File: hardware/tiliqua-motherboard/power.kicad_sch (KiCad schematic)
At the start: 23 parts, among them J6 CONN 2x5 P=2.54mm, U5 AP63200WU

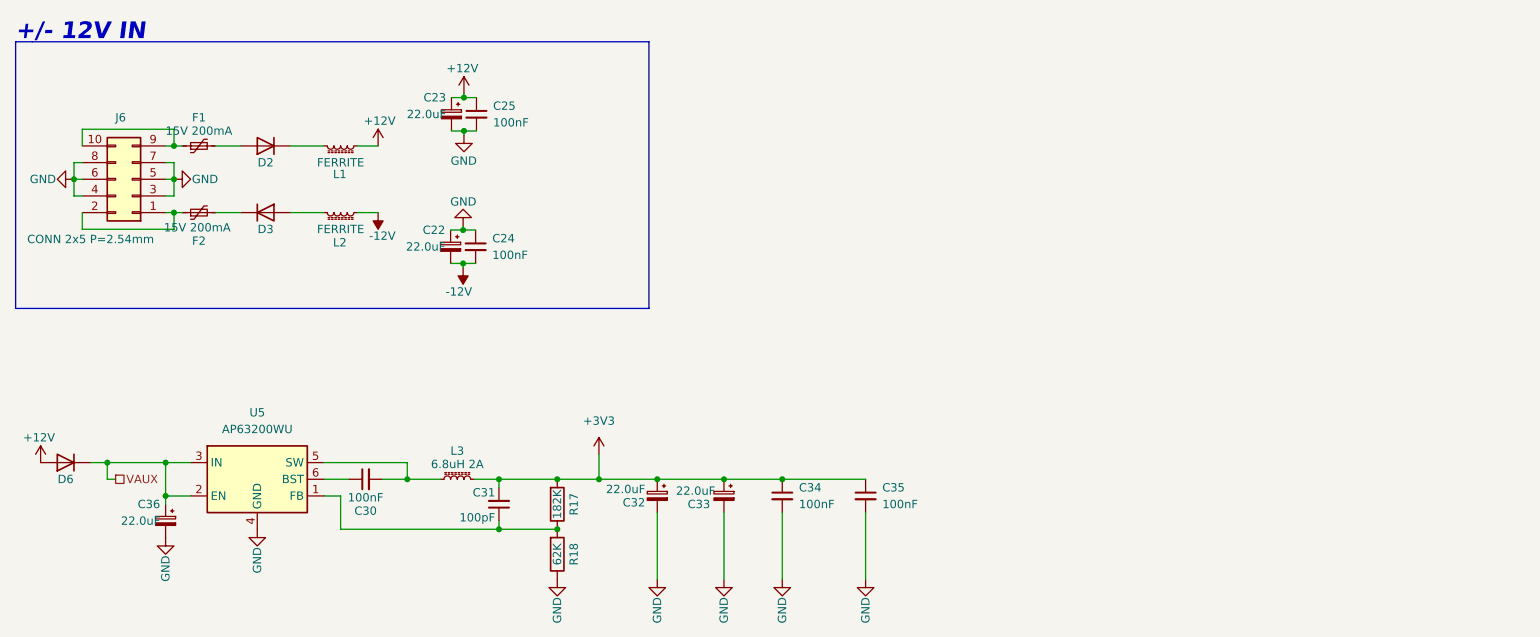
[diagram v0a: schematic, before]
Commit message: R2 start
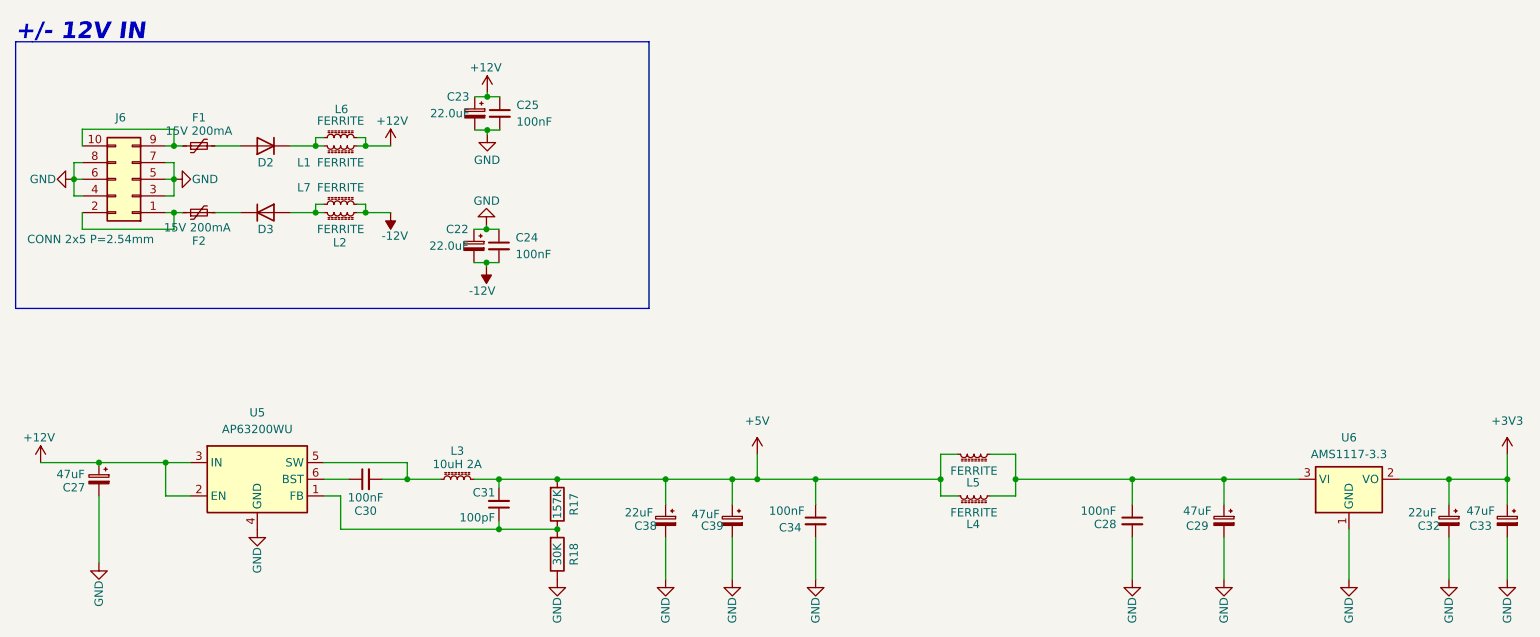
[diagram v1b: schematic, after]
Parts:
- removed C35: 100nF, Capacitor_SMD:C_0603_1608Metric, symbol Device:C_Small
- removed C36: 22.0uF, Capacitor_Tantalum_SMD:CP_EIA-3216-10_Kemet-I, symbol Device:C_Polarized_Small
- removed D6: 1N4007FL, Diode_SMD:D_SOD-123F, symbol Diode:US1G
- added C27, C29, C39: 47uF, Capacitor_SMD:CP_Elec_6.3x5.4, symbol Device:C_Polarized_Small
- added C28: 100nF, Capacitor_SMD:C_0603_1608Metric, symbol Device:C_Small
- added C38: 22uF, Capacitor_Tantalum_SMD:CP_EIA-3216-10_Kemet-I, symbol Device:C_Polarized_Small
- added L4, L5, L6, L7: FERRITE, Inductor_SMD:L_0603_1608Metric, symbol Device:L_Ferrite_Small
- added U6: AMS1117-3.3, Package_TO_SOT_SMD:SOT-223-3_TabPin2, symbol Regulator_Linear:AMS1117-3.3
- C32: value 22.0uF -> 22uF
- C33: value 22.0uF -> 47uF; footprint Capacitor_Tantalum_SMD:CP_EIA-3216-10_Kemet-I -> Capacitor_SMD:CP_Elec_6.3x5.4; lcsc# C782264 -> C88735; mfg# CA45-A-16V-22uF-K -> 25SEV47M6.3X5.5
- L3: value 6.8uH 2A -> 10uH 2A; lcsc# C844992 -> (none)
- R17: value 182K -> 157K; PN RC0402FR-074K7L -> (none); lcsc# C327365 -> (none)
- R18: value 62K -> 30K; PN RC0402FR-074K7L -> (none); lcsc# C137950 -> (none)
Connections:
- net VAUX is gone; now on net +12V: U5.2 (EN), U5.3 (IN)
- net +12V: now also C27.1, L6.2
- net +3V3: now also U6.2 (VO); no longer C31.2, C34.1, L3.2, R17.2
- net -12V: now also L7.2
- net GND: now also C27.2, C28.2, C29.2, C38.2, C39.2, U6.1 (GND)
- net at D3.2 (A), L2.2: now also L7.1
- net at D2.1 (K), L1.2: now also L6.1
- new net: C28.1, C29.1, L4.1, L5.1, U6.3 (VI)
- new net +5V: C31.2, C34.1, C38.1, C39.1, L3.2, L4.2, L5.2, R17.2
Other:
- moved on the sheet: C22, C23, C24, C25, C34
